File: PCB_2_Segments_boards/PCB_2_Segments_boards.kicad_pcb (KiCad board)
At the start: 2 copper layers, 2 parts

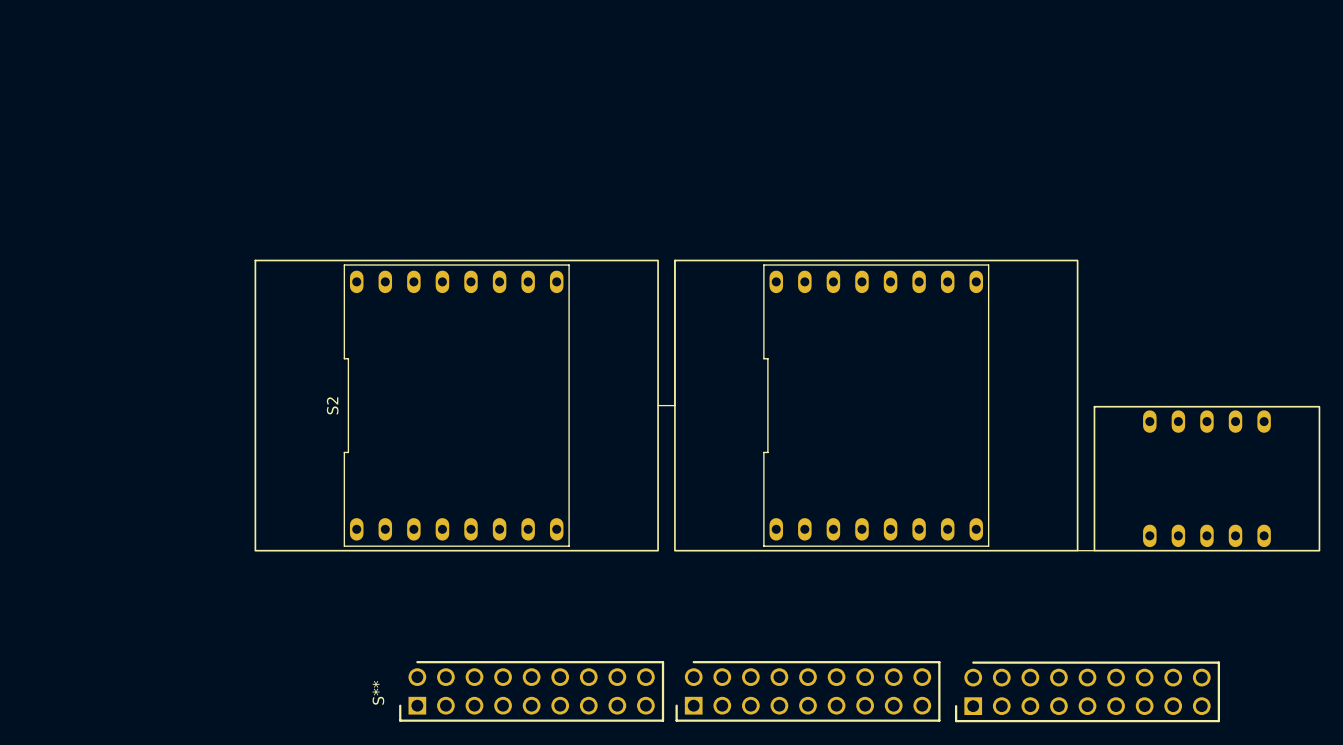
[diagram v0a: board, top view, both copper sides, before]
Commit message: backup update
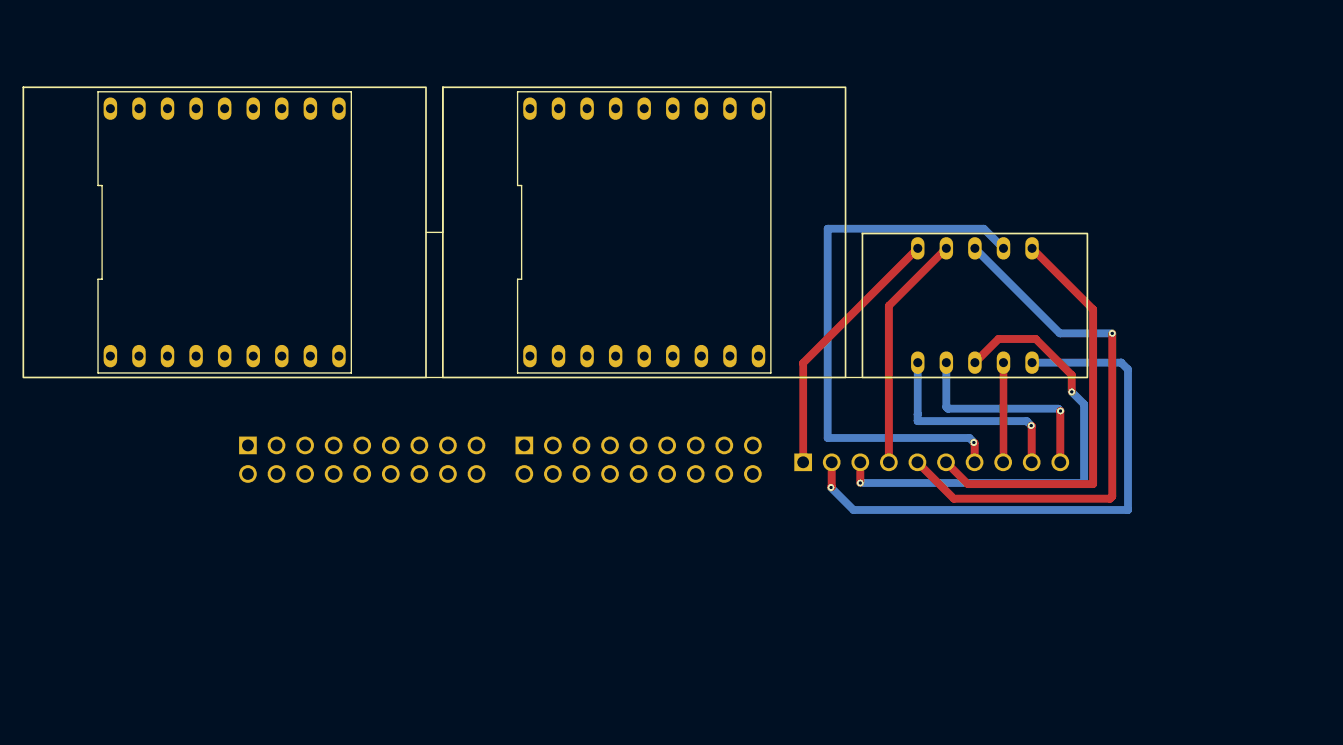
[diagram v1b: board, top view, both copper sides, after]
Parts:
- S1: moved to B.Cu
- moved S2 25.7 mm to (100.2, 81.5)
- moved S1 25.1 mm to (111.9, 102.0), turned to -90 degrees
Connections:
- S1 pad 1: unconnected-(S1-Pad1) -> Net-(S1-Pad1)
- S1 pad 10: unconnected-(S1-Pad10) -> Net-(S1-Pad10)
- S1 pad 11: unconnected-(S1-Pad11) -> Net-(S1-Pad11)
- S1 pad 12: unconnected-(S1-Pad12) -> Net-(S1-Pad12)
- S1 pad 13: unconnected-(S1-Pad13) -> Net-(S1-Pad13)
- S1 pad 14: unconnected-(S1-Pad14) -> Net-(S1-Pad14)
- S1 pad 15: unconnected-(S1-Pad15) -> Net-(S1-Pad15)
- S1 pad 16: unconnected-(S1-Pad16) -> Net-(S1-Pad16)
- S1 pad 17: unconnected-(S1-Pad17) -> Net-(S1-Pad17)
- S1 pad 18: unconnected-(S1-Pad18) -> Net-(S1-Pad18)
- S1 pad 19: unconnected-(S1-Pad19) -> Net-(S1-Pad19)
- S1 pad 2: unconnected-(S1-Pad2) -> Net-(S1-Pad2)
- S1 pad 20: unconnected-(S1-Pad20) -> Net-(S1-Pad20)
- S1 pad 21: unconnected-(S1-Pad21) -> Net-(S1-Pad21)
- S1 pad 22: unconnected-(S1-Pad22) -> Net-(S1-Pad22)
- S1 pad 23: unconnected-(S1-Pad23) -> Net-(S1-Pad23)
- S1 pad 24: unconnected-(S1-Pad24) -> Net-(S1-Pad24)
- S1 pad 25: unconnected-(S1-Pad25) -> Net-(S1-Pad25)
- S1 pad 26: unconnected-(S1-Pad26) -> Net-(S1-Pad26)
- S1 pad 27: unconnected-(S1-Pad27) -> Net-(S1-Pad27)
- S1 pad 28: unconnected-(S1-Pad28) -> Net-(S1-Pad28)
- S1 pad 29: unconnected-(S1-Pad29) -> Net-(S1-Pad29)
- S1 pad 3: unconnected-(S1-Pad3) -> Net-(S1-Pad3)
- S1 pad 30: unconnected-(S1-Pad30) -> Net-(S1-Pad30)
- S1 pad 31: unconnected-(S1-Pad31) -> Net-(S1-Pad31)
- S1 pad 32: unconnected-(S1-Pad32) -> Net-(S1-Pad32)
- S1 pad 33: unconnected-(S1-Pad33) -> Net-(S1-Pad33)
- S1 pad 34: unconnected-(S1-Pad34) -> Net-(S1-Pad34)
- S1 pad 35: unconnected-(S1-Pad35) -> Net-(S1-Pad35)
- S1 pad 36: unconnected-(S1-Pad36) -> Net-(S1-Pad36)
- S1 pad 37: unconnected-(S1-Pad37) -> Net-(S1-Pad37)
- S1 pad 38: unconnected-(S1-Pad38) -> Net-(S1-Pad38)
- S1 pad 39: unconnected-(S1-Pad39) -> Net-(S1-Pad39)
- S1 pad 4: unconnected-(S1-Pad4) -> Net-(S1-Pad4)
- S1 pad 40: unconnected-(S1-Pad40) -> Net-(S1-Pad40)
- S1 pad 41: unconnected-(S1-Pad41) -> Net-(S1-Pad41)
- S1 pad 42: unconnected-(S1-Pad42) -> Net-(S1-Pad42)
- S1 pad 43: unconnected-(S1-Pad43) -> Net-(S1-Pad43)
- S1 pad 44: unconnected-(S1-Pad44) -> Net-(S1-Pad44)
- S1 pad 45: unconnected-(S1-Pad45) -> Net-(S1-Pad45)
- S1 pad 46: unconnected-(S1-Pad46) -> Net-(S1-Pad46)
- S1 pad 5: unconnected-(S1-Pad5) -> Net-(S1-Pad5)
- S1 pad 6: unconnected-(S1-Pad6) -> Net-(S1-Pad6)
- S1 pad 7: unconnected-(S1-Pad7) -> Net-(S1-Pad7)
- S1 pad 8: unconnected-(S1-Pad8) -> Net-(S1-Pad8)
- S1 pad 9: unconnected-(S1-Pad9) -> Net-(S1-Pad9)
- S2 pad 1: unconnected-(S2-Pad1) -> Net-(S1-Pad1)
- S2 pad 10: unconnected-(S2-Pad10) -> Net-(S1-Pad10)
- S2 pad 11: unconnected-(S2-Pad11) -> Net-(S1-Pad11)
- S2 pad 12: unconnected-(S2-Pad12) -> Net-(S1-Pad12)
- S2 pad 13: unconnected-(S2-Pad13) -> Net-(S1-Pad13)
- S2 pad 14: unconnected-(S2-Pad14) -> Net-(S1-Pad14)
- S2 pad 15: unconnected-(S2-Pad15) -> Net-(S1-Pad15)
- S2 pad 16: unconnected-(S2-Pad16) -> Net-(S1-Pad16)
- S2 pad 17: unconnected-(S2-Pad17) -> Net-(S1-Pad17)
- S2 pad 18: unconnected-(S2-Pad18) -> Net-(S1-Pad18)
- S2 pad 19: unconnected-(S2-Pad19) -> Net-(S1-Pad19)
- S2 pad 2: unconnected-(S2-Pad2) -> Net-(S1-Pad2)
- S2 pad 20: unconnected-(S2-Pad20) -> Net-(S1-Pad20)
- S2 pad 21: unconnected-(S2-Pad21) -> Net-(S1-Pad21)
- S2 pad 22: unconnected-(S2-Pad22) -> Net-(S1-Pad22)
- S2 pad 23: unconnected-(S2-Pad23) -> Net-(S1-Pad23)
- S2 pad 24: unconnected-(S2-Pad24) -> Net-(S1-Pad24)
- S2 pad 25: unconnected-(S2-Pad25) -> Net-(S1-Pad25)
- S2 pad 26: unconnected-(S2-Pad26) -> Net-(S1-Pad26)
- S2 pad 27: unconnected-(S2-Pad27) -> Net-(S1-Pad27)
- S2 pad 28: unconnected-(S2-Pad28) -> Net-(S1-Pad28)
- S2 pad 29: unconnected-(S2-Pad29) -> Net-(S1-Pad29)
- S2 pad 3: unconnected-(S2-Pad3) -> Net-(S1-Pad3)
- S2 pad 30: unconnected-(S2-Pad30) -> Net-(S1-Pad30)
- S2 pad 31: unconnected-(S2-Pad31) -> Net-(S1-Pad31)
- S2 pad 32: unconnected-(S2-Pad32) -> Net-(S1-Pad32)
- S2 pad 33: unconnected-(S2-Pad33) -> Net-(S1-Pad33)
- S2 pad 34: unconnected-(S2-Pad34) -> Net-(S1-Pad34)
- S2 pad 35: unconnected-(S2-Pad35) -> Net-(S1-Pad35)
- S2 pad 36: unconnected-(S2-Pad36) -> Net-(S1-Pad36)
- S2 pad 37: unconnected-(S2-Pad37) -> Net-(S1-Pad37)
- S2 pad 38: unconnected-(S2-Pad38) -> Net-(S1-Pad38)
- S2 pad 39: unconnected-(S2-Pad39) -> Net-(S1-Pad39)
- S2 pad 4: unconnected-(S2-Pad4) -> Net-(S1-Pad4)
- S2 pad 40: unconnected-(S2-Pad40) -> Net-(S1-Pad40)
- S2 pad 41: unconnected-(S2-Pad41) -> Net-(S1-Pad41)
- S2 pad 42: unconnected-(S2-Pad42) -> Net-(S1-Pad42)
- S2 pad 5: unconnected-(S2-Pad5) -> Net-(S1-Pad5)
- S2 pad 6: unconnected-(S2-Pad6) -> Net-(S1-Pad6)
- S2 pad 7: unconnected-(S2-Pad7) -> Net-(S1-Pad7)
- S2 pad 8: unconnected-(S2-Pad8) -> Net-(S1-Pad8)
- S2 pad 9: unconnected-(S2-Pad9) -> Net-(S1-Pad9)
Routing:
- net Net-(S1-Pad20): track 0.00 -> 50.8 mm, vias 0 -> 1
- net Net-(S1-Pad25): track 0.00 -> 49.9 mm, vias 0 -> 1
- net Net-(S1-Pad23): track 0.00 -> 48.6 mm, vias 0 -> 1
- net Net-(S1-Pad21): track 0.00 -> 42.6 mm, vias 0 -> 2
- net Net-(S1-Pad24): track 0.00 -> 37.1 mm
- net Net-(S1-Pad19): track 0.00 -> 23.2 mm
- net Net-(S1-Pad22): track 0.00 -> 21.1 mm
- net Net-(S1-Pad28): track 0.00 -> 18.8 mm, vias 0 -> 1
- net Net-(S1-Pad27): track 0.00 -> 18.7 mm, vias 0 -> 1
- net Net-(S1-Pad26): track 0.00 -> 8.87 mm

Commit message: backup update
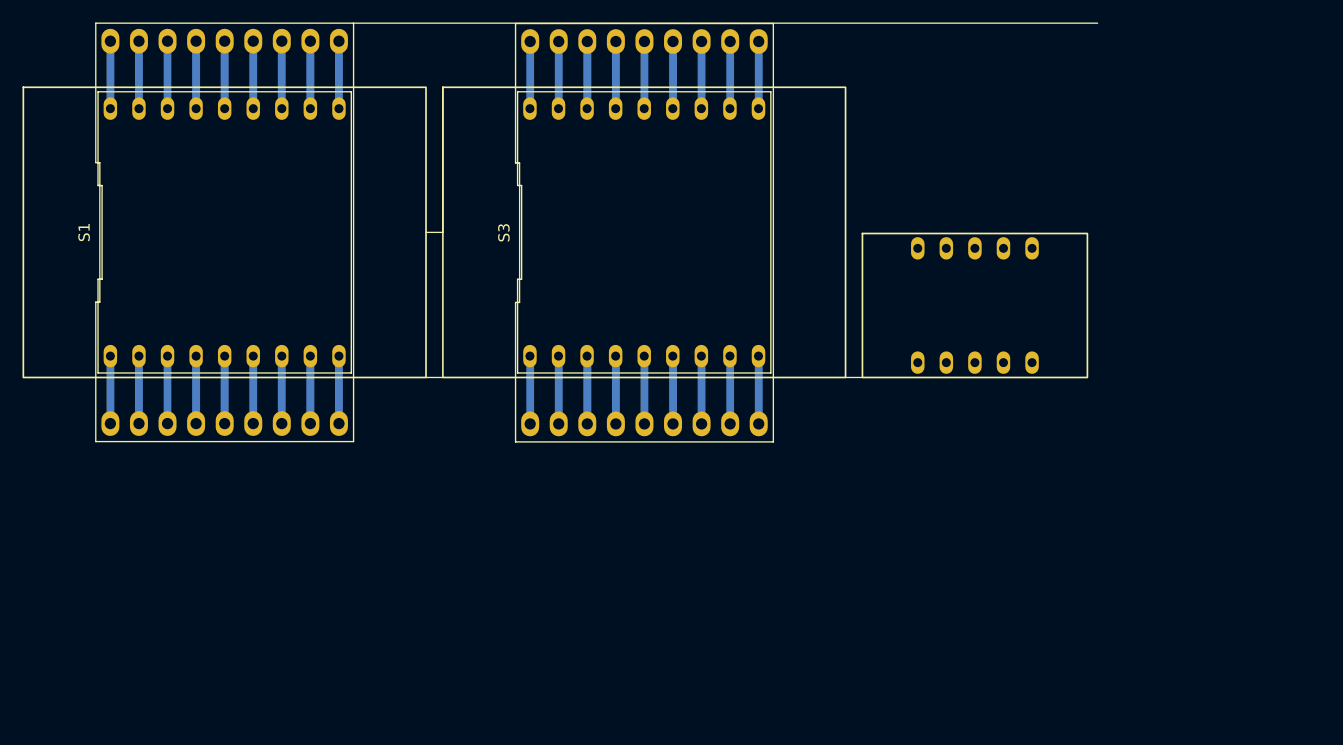
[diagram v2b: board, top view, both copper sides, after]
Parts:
- added S3: ~, My parts:DIP 18 Patice Display Digit 2, F.Cu at (137.5, 81.5)
- S1: value S -> ~; footprint My parts:Screen_connector_footprint -> My parts:DIP 18 Patice Display Digit 1; moved to F.Cu
- moved S1 23.6 mm to (100.2, 81.5), turned to 0 degrees
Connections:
- S2 pad 10: Net-(S1-Pad10) -> Net-(S2-Pad10)
- S2 pad 11: Net-(S1-Pad11) -> Net-(S2-Pad11)
- S2 pad 12: Net-(S1-Pad12) -> Net-(S2-Pad12)
- S2 pad 13: Net-(S1-Pad13) -> Net-(S2-Pad13)
- S2 pad 14: Net-(S1-Pad14) -> Net-(S2-Pad14)
- S2 pad 15: Net-(S1-Pad15) -> Net-(S2-Pad15)
- S2 pad 16: Net-(S1-Pad16) -> Net-(S2-Pad16)
- S2 pad 17: Net-(S1-Pad17) -> Net-(S2-Pad17)
- S2 pad 18: Net-(S1-Pad18) -> Net-(S2-Pad18)
- S2 pad 19: Net-(S1-Pad19) -> Net-(S2-Pad19)
- S2 pad 20: Net-(S1-Pad20) -> Net-(S2-Pad20)
- S2 pad 21: Net-(S1-Pad21) -> Net-(S2-Pad21)
- S2 pad 22: Net-(S1-Pad22) -> Net-(S2-Pad22)
- S2 pad 23: Net-(S1-Pad23) -> Net-(S2-Pad23)
- S2 pad 24: Net-(S1-Pad24) -> Net-(S2-Pad24)
- S2 pad 25: Net-(S1-Pad25) -> Net-(S2-Pad25)
- S2 pad 26: Net-(S1-Pad26) -> Net-(S2-Pad26)
- S2 pad 27: Net-(S1-Pad27) -> Net-(S2-Pad27)
- S2 pad 28: Net-(S1-Pad28) -> Net-(S2-Pad28)
- S2 pad 29: Net-(S1-Pad29) -> Net-(S2-Pad29)
- S2 pad 30: Net-(S1-Pad30) -> Net-(S2-Pad30)
- S2 pad 31: Net-(S1-Pad31) -> Net-(S2-Pad31)
- S2 pad 32: Net-(S1-Pad32) -> Net-(S2-Pad32)
- S2 pad 33: Net-(S1-Pad33) -> Net-(S2-Pad33)
- S2 pad 34: Net-(S1-Pad34) -> Net-(S2-Pad34)
- S2 pad 35: Net-(S1-Pad35) -> Net-(S2-Pad35)
- S2 pad 36: Net-(S1-Pad36) -> Net-(S2-Pad36)
- S2 pad 37: Net-(S1-Pad37) -> Net-(S2-Pad37)
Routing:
- net Net-(S1-Pad20): track 50.8 -> 0.00 mm, vias 1 -> 0
- net Net-(S1-Pad25): track 49.9 -> 0.00 mm, vias 1 -> 0
- net Net-(S1-Pad23): track 48.6 -> 0.00 mm, vias 1 -> 0
- net Net-(S1-Pad21): track 42.6 -> 0.00 mm, vias 2 -> 0
- net Net-(S1-Pad24): track 37.1 -> 0.00 mm
- net Net-(S1-Pad19): track 23.2 -> 0.00 mm
- net Net-(S1-Pad22): track 21.1 -> 0.00 mm
- net Net-(S1-Pad28): track 18.8 -> 0.00 mm, vias 1 -> 0
- net Net-(S1-Pad27): track 18.7 -> 0.00 mm, vias 1 -> 0
- net Net-(S1-Pad26): track 8.87 -> 0.00 mm
- net Net-(S1-Pad40): track 0.00 -> 6.38 mm
- net Net-(S2-Pad33): track 0.00 -> 6.04 mm
- net Net-(S2-Pad30): track 0.00 -> 6.04 mm
- net Net-(S2-Pad18): track 0.00 -> 6.04 mm
- net Net-(S2-Pad13): track 0.00 -> 6.04 mm
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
